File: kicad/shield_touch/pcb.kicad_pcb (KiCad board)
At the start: 2 copper layers, 48.9 x 49.5 mm, 22 parts, among them J1 Conn_01x12_Fem_l, J2 Conn_01x12_Fem_r, J3 Conn_01x09_Fem_b_l, J4 Conn_01x11_Fem_b_r_touch

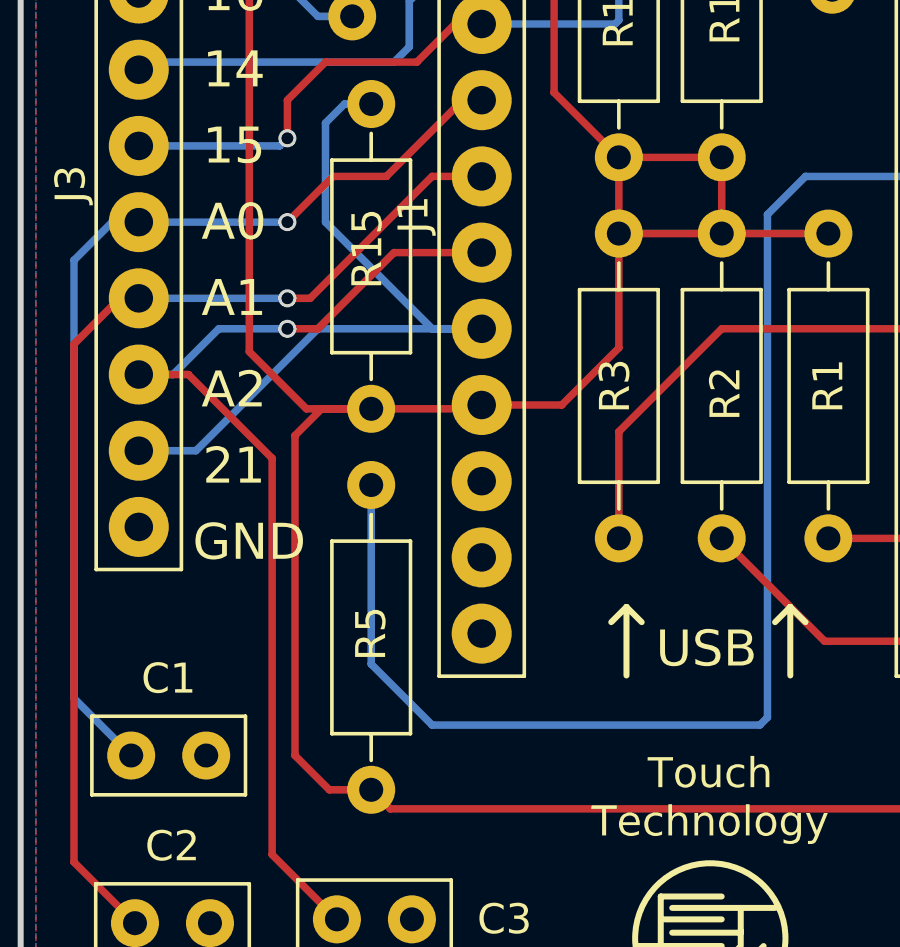
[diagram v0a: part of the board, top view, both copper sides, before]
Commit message: update
- still to fix
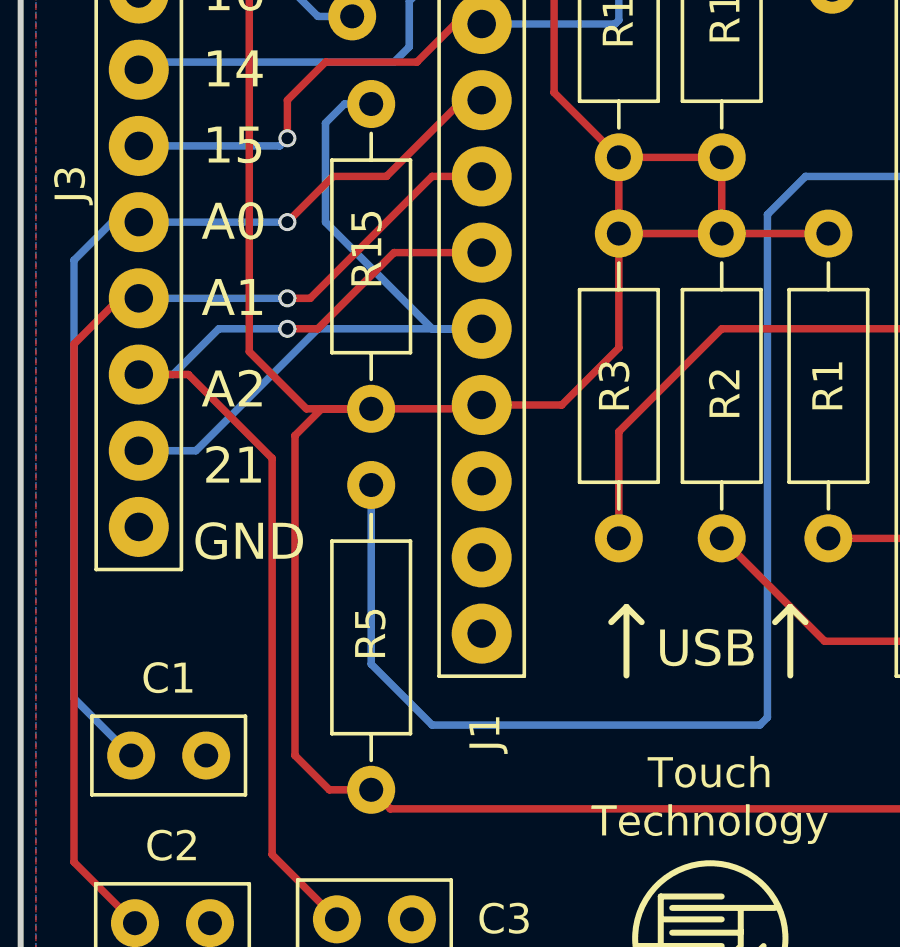
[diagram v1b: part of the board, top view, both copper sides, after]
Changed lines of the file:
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@@
   (page A4)
   (layers
-    (0 F.Cu signal hide)
-    (31 B.Cu signal hide)
+    (0 F.Cu signal)
+    (31 B.Cu signal)
     (32 B.Adhes user)
     (33 F.Adhes user)
     (34 B.Paste user)
     (35 F.Paste user)
-    (36 B.SilkS user hide)
+    (36 B.SilkS user)
     (37 F.SilkS user)
     (38 B.Mask user)
@@
     (descr "Low profile, screw machine socket strip, through hole, 100mil / 2.54mm pitch")
     (tags "samtec socket strip tht single")
-    (fp_text reference J1 (at -2.27 13.97 90) (layer F.SilkS)
-      (effects (font (size 1 1) (thickness 0.15)))
-    )
+    (fp_text reference J1 (at 0.127 31.242 90) (layer F.SilkS)
+      (effects (font (size 1 1) (thickness 0.15)))
+    )
